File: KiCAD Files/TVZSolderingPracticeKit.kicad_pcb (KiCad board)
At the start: 2 copper layers, 108 x 108 mm, 28 parts, among them J1 Barrel Jack, SW1 SW_Push, SW10 SW_SPDT, SW2 SW_Push, SW3 SW_Push, SW4 SW_Push, SW5 SW_Push, SW6 SW_Push, SW7 SW_Push, SW8 SW_Push, U1 NE555P

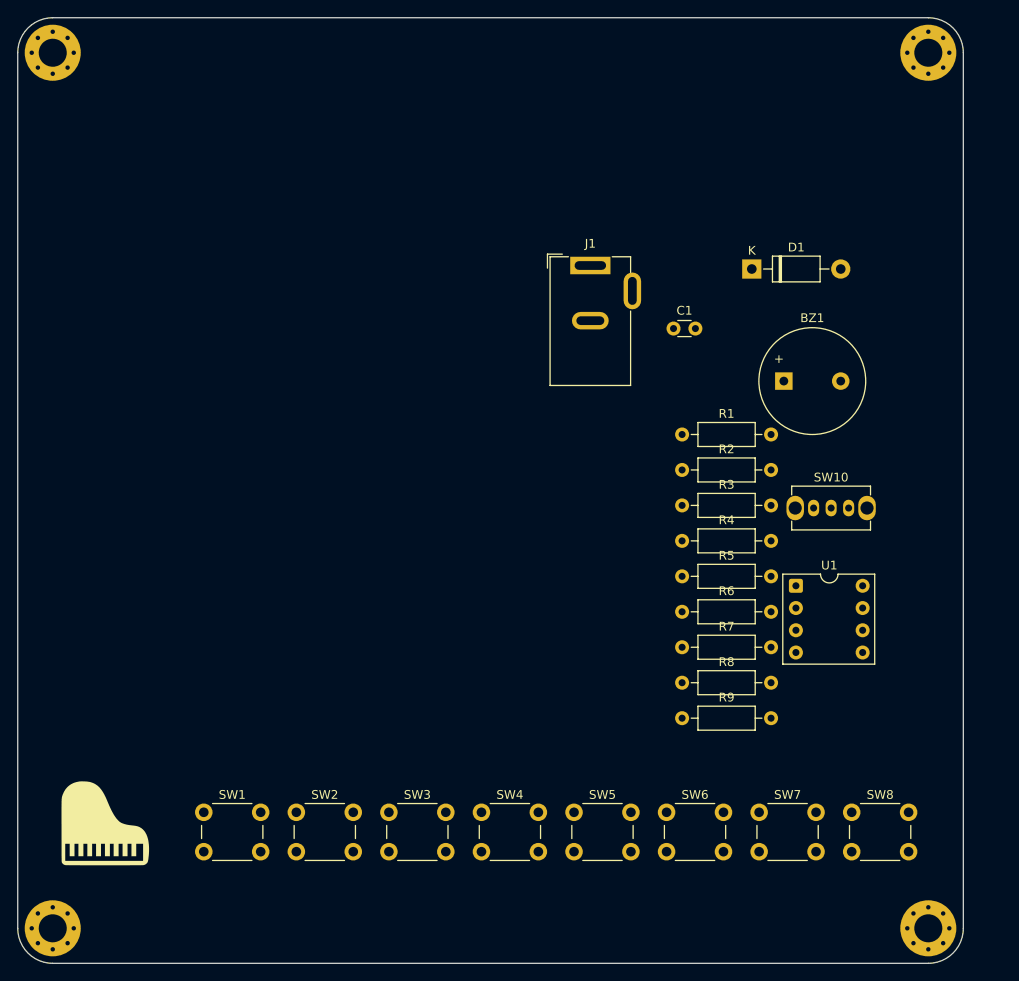
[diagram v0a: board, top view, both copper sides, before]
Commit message: update
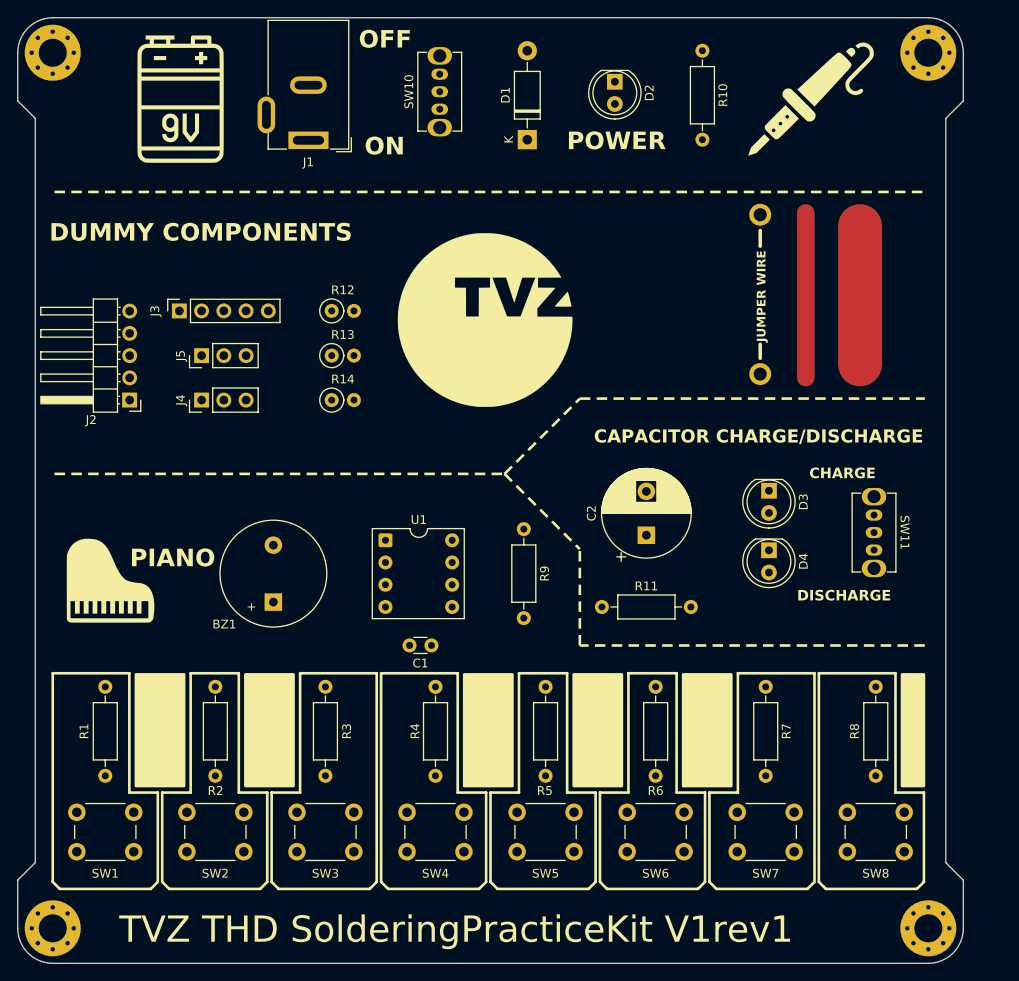
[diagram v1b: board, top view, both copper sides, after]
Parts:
- added C2: 470u / 50V, Capacitor_THT:CP_Radial_D10.0mm_P5.00mm, F.Cu at (117.8, 135.6)
- added D2: RED, LED_THT:LED_D5.0mm, F.Cu at (114.2, 83.8)
- added D3: YELLOW, LED_THT:LED_D5.0mm, F.Cu at (131.8, 130.5)
- added D4: GREEN, LED_THT:LED_D5.0mm, F.Cu at (131.8, 137.3)
- added G***: LOGO, Footprint:9V, F.Cu at (64.6, 85.8)
- added G***: LOGO, Footprint:soldering, F.Cu at (136.6, 85.8)
- added G***: LOGO, Footprint:TVZ, F.Cu at (99.4, 111.0)
- added J2: Conn_01x05_Pin, Connector_PinHeader_2.54mm:PinHeader_1x05_P2.54mm_Horizontal, F.Cu at (58.8, 120.2)
- added J3: Conn_01x05_Socket, Connector_PinSocket_2.54mm:PinSocket_1x05_P2.54mm_Vertical, F.Cu at (64.5, 110.0)
- added J4: Conn_01x03_Pin, Connector_PinHeader_2.54mm:PinHeader_1x03_P2.54mm_Vertical, F.Cu at (67.0, 120.2)
- added J5: Conn_01x03_Pin, Connector_PinHeader_2.54mm:PinHeader_1x03_P2.54mm_Vertical, F.Cu at (67.0, 115.1)
- added R10: 4k7, Resistor_THT:R_Axial_DIN0207_L6.3mm_D2.5mm_P10.16mm_Horizontal, F.Cu at (124.2, 80.3)
- added R11: 2k2, Resistor_THT:R_Axial_DIN0207_L6.3mm_D2.5mm_P10.16mm_Horizontal, F.Cu at (112.7, 143.8)
- added R12: 2k2, Resistor_THT:R_Axial_DIN0207_L6.3mm_D2.5mm_P2.54mm_Vertical, F.Cu at (81.9, 110.0)
- added R13: 2k2, Resistor_THT:R_Axial_DIN0207_L6.3mm_D2.5mm_P2.54mm_Vertical, F.Cu at (81.9, 115.1)
- added R14: 2k2, Resistor_THT:R_Axial_DIN0207_L6.3mm_D2.5mm_P2.54mm_Vertical, F.Cu at (81.9, 120.2)
- added SW11: C/D, Footprint:OS102011MS2QN1, F.Cu at (143.8, 135.3)
- added TP1: TestPoint, Footprint:Wire, F.Cu at (130.8, 99.0)
- added TP2: TestPoint, Footprint:Wire, F.Cu at (130.8, 117.2)
- SW10: value SW_SPDT -> POWER
- moved R1 65.9 mm to (56.0, 152.9), turned to -90 degrees
- moved SW10 65.3 mm to (94.2, 85.0), turned to 90 degrees
- moved BZ1 63.5 mm to (75.2, 143.2), turned to 90 degrees
- moved R2 53.5 mm to (68.6, 152.9), turned to -90 degrees
- moved U1 47.2 mm to (88.0, 136.2)
- moved C1 45.5 mm to (93.2, 148.2), turned to 180 degrees
- moved R3 41.6 mm to (81.1, 152.9), turned to -90 degrees
- moved R8 36.3 mm to (144.0, 152.9), turned to -90 degrees
- moved J1 35.2 mm to (79.2, 90.5), turned to 180 degrees
- moved R4 30.9 mm to (93.7, 152.9), turned to -90 degrees
- moved D1 29.6 mm to (104.2, 90.4), turned to 90 degrees
- moved G*** 27.7 mm to (56.6, 140.8)
- moved R7 26.5 mm to (131.4, 152.9), turned to -90 degrees
- moved R5 22.8 mm to (106.3, 152.9), turned to -90 degrees
- moved R9 21.4 mm to (103.8, 145.1), turned to 90 degrees
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- renumbered R8 to R1, R7 to R2, R6 to R3, R5 to R4, R4 to R5, R3 to R6, R2 to R7, R1 to R8
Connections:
- net Net-(D1-K) renamed VDD
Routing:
- net (no net): track 0.00 -> 34.6 mm
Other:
- outline, holes or cut-outs redrawn
- board text added: "CAPACITOR CHARGE/DISCHARGE"
- board text added: "CHARGE"
- board text added: "DISCHARGE"
- board text added: "DUMMY COMPONENTS"
- board text added: "JUMPER WIRE"
- board text added: "OFF"
- board text added: "ON"
- board text added: "PIANO"
- board text added: "POWER"
- board text added: "TVZ THD SolderingPracticeKit V1rev1"
